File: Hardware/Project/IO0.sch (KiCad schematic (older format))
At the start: 1 part, among them U6 8255

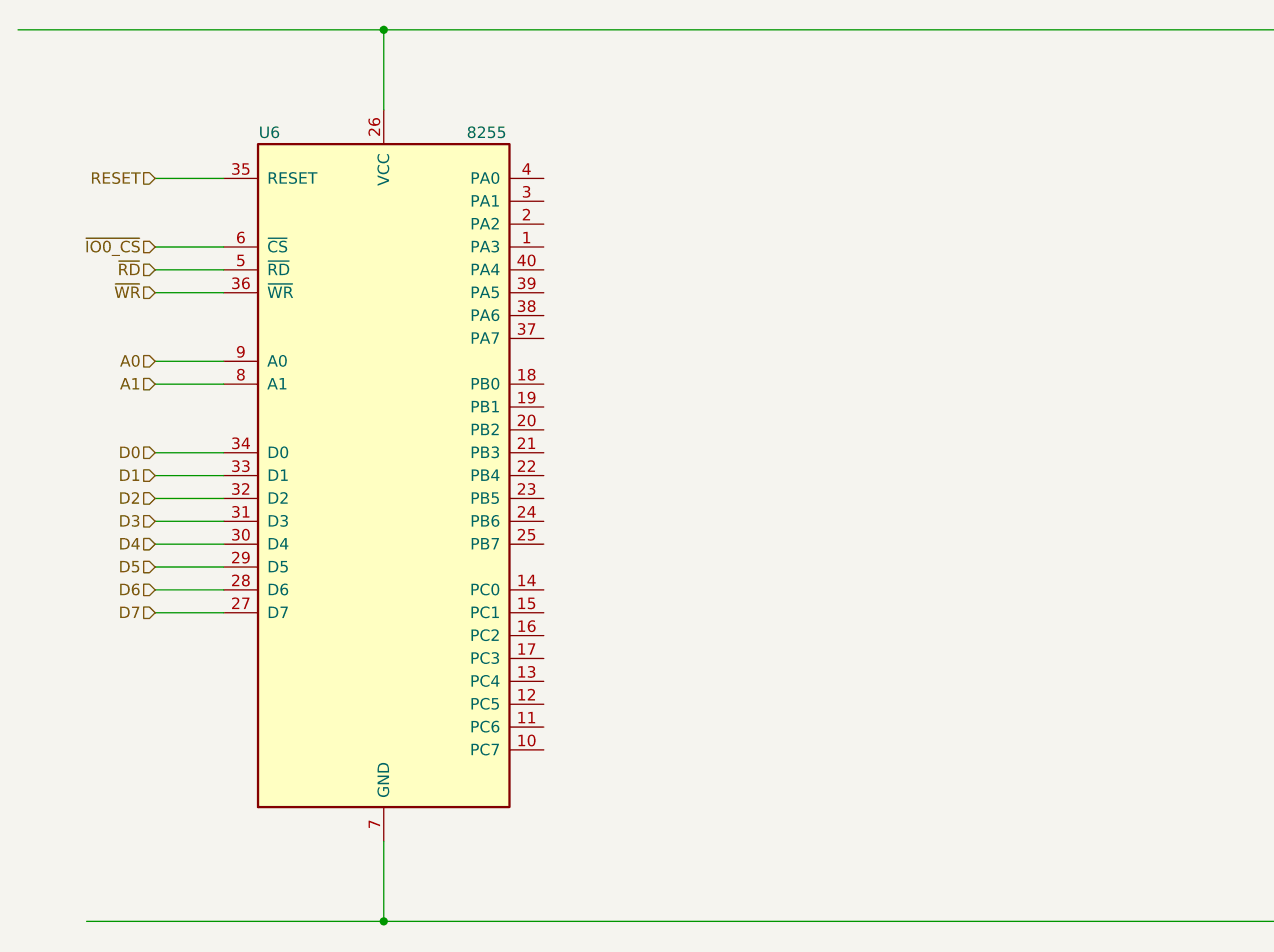
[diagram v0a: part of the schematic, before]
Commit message: 1
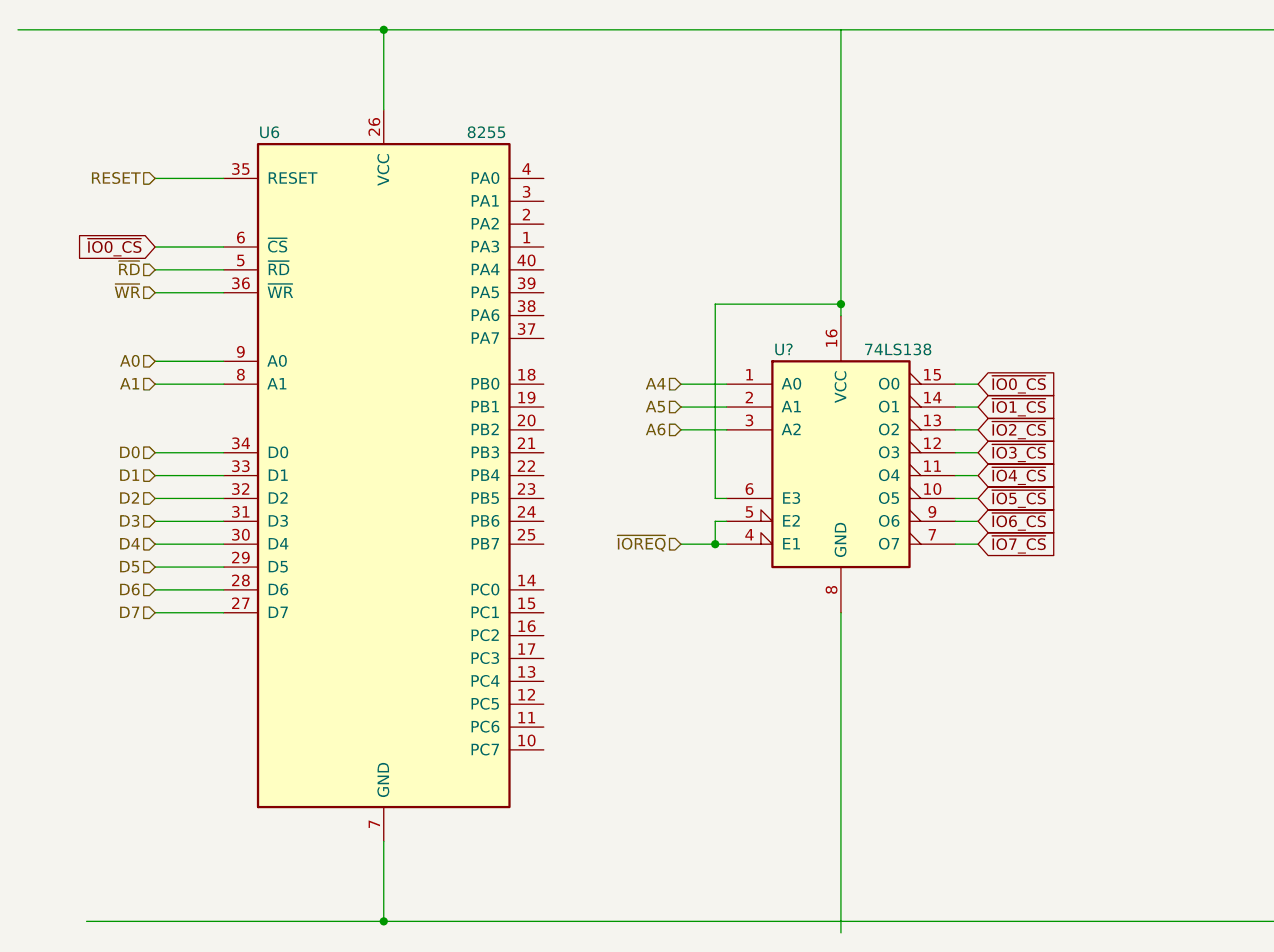
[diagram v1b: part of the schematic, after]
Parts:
- added U?: 74LS138, symbol 74xx:74LS138
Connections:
- net labels added: A4, A5, A6, ~IO1_CS, ~IO2_CS, ~IO3_CS, ~IO4_CS, ~IO5_CS, ~IO6_CS, ~IO7_CS, ~IOREQ
- wire segments 20 -> 41
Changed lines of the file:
@@
 EESchema Schematic File Version 4
+LIBS:8051-cache
 EELAYER 26 0
 EELAYER END
 $Descr A3 16535 11693
 encoding utf-8
-Sheet 3 5
+Sheet 3 6
 Title ""
 Date ""
@@
 AR Path="/5DFCE73E/5DEE654C" Ref="U?"  Part="1"
 AR Path="/5E02D9A0/5DEE654C" Ref="U?"  Part="1"
+AR Path="/5D59EC5C/5DEE654C" Ref="U?"  Part="1"
+AR Path="/5D62F4AC/5DEE654C" Ref="U?"  Part="1"
 F 0 "U6" H 2250 4600 50  0000 C CNN
 F 1 "8255" H 3200 4600 50  0000 C CNN
@@
 Wire Wire Line
 	2050 2300 1750 2300
-Text HLabel 1750 2100 0    50   Input ~ 0
-~IO0_CS
 Wire Wire Line
 	2050 2100 1750 2100
@@
 Wire Wire Line
 	2050 1800 1750 1800
+$Comp
+L 74xx:74LS138 U?
+U 1 1 5D4417B6
+P 4750 3000
+AR Path="/5C68B4BB/5D4417B6" Ref="U?"  Part="1"
+AR Path="/5DED3C2A/5D4417B6" Ref="U?"  Part="1"
+AR Path="/5D59EC5C/5D4417B6" Ref="U?"  Part="1"
+AR Path="/5D62F4AC/5D4417B6" Ref="U?"  Part="1"
+F 0 "U?" H 4500 3450 50  0000 C CNN
+F 1 "74LS138" H 5000 3450 50  0000 C CNN
+F 2 "" H 4750 3000 50  0001 C CNN
+F 3 "http://www.ti.com/lit/gpn/sn74LS138" H 4750 3000 50  0001 C CNN
+	1    4750 3000
+	1    0    0    -1
+$EndComp
+Wire Wire Line
+	4750 2400 4750 2350
+Wire Wire Line
+	4750 3700 4750 5100
+Text HLabel 4050 2900 0    50   Input ~ 0
+A6
+Text HLabel 4050 2800 0    50   Input ~ 0
+A5
+Text HLabel 4050 2700 0    50   Input ~ 0
+A4
+Wire Wire Line
+	4250 2700 4050 2700
+Wire Wire Line
+	4250 2800 4050 2800
+Wire Wire Line
+	4250 2900 4050 2900
+Wire Wire Line
+	4250 3300 4200 3300
+Wire Wire Line
+	4200 3300 4200 3400
+Wire Wire Line
+	4200 3400 4250 3400
+Wire Wire Line
+	4250 3200 4200 3200
+Wire Wire Line
+	4200 3200 4200 2350
+Wire Wire Line
+	4200 2350 4750 2350
+Connection ~ 4750 2350
+Wire Wire Line
+	4750 2350 4750 1150
+Text GLabel 5350 2700 2    50   Input ~ 0
+~IO0_CS
+Connection ~ 4200 3400
+Wire Wire Line
+	5350 2700 5250 2700
+Text HLabel 4050 3400 0    50   Input ~ 0
+~IOREQ
+Wire Wire Line
+	4050 3400 4200 3400
+Text GLabel 5350 2800 2    50   Input ~ 0
+~IO1_CS
+Wire Wire Line
+	5350 2800 5250 2800
+Text GLabel 5350 2900 2    50   Input ~ 0
+~IO2_CS
+Wire Wire Line
+	5350 2900 5250 2900
+Text GLabel 5350 3000 2    50   Input ~ 0
+~IO3_CS
+Wire Wire Line
+	5350 3000 5250 3000
+Text GLabel 5350 3100 2    50   Input ~ 0
+~IO4_CS
+Wire Wire Line
+	5350 3100 5250 3100
+Text GLabel 5350 3200 2    50   Input ~ 0
+~IO5_CS
+Wire Wire Line
+	5350 3200 5250 3200
+Text GLabel 5350 3300 2    50   Input ~ 0
+~IO6_CS
+Wire Wire Line
+	5350 3300 5250 3300
+Text GLabel 5350 3400 2    50   Input ~ 0
+~IO7_CS
+Wire Wire Line
+	5350 3400 5250 3400
+Text GLabel 1750 2100 0    50   Input ~ 0
+~IO0_CS
 $EndSCHEMATC
